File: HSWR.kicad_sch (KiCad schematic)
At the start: 25 parts, among them J1 IO, J10 W2, J2 USB_B, J3 B+, J4 B-, J5 U1, J6 V1, J7 W1, J8 U2, J9 V2, U14 Opamp_Quad

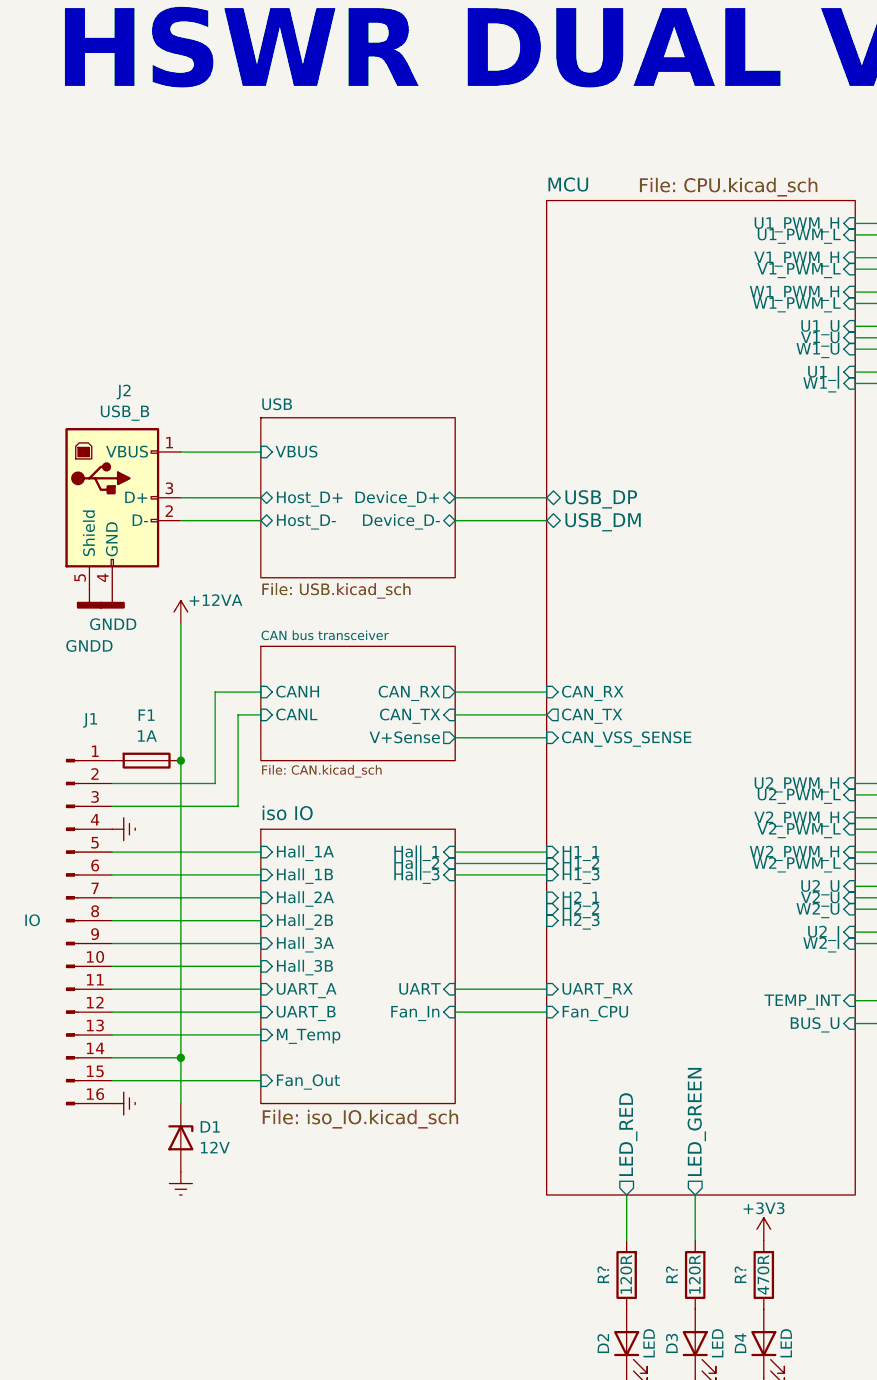
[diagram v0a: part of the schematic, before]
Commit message: - some layout work
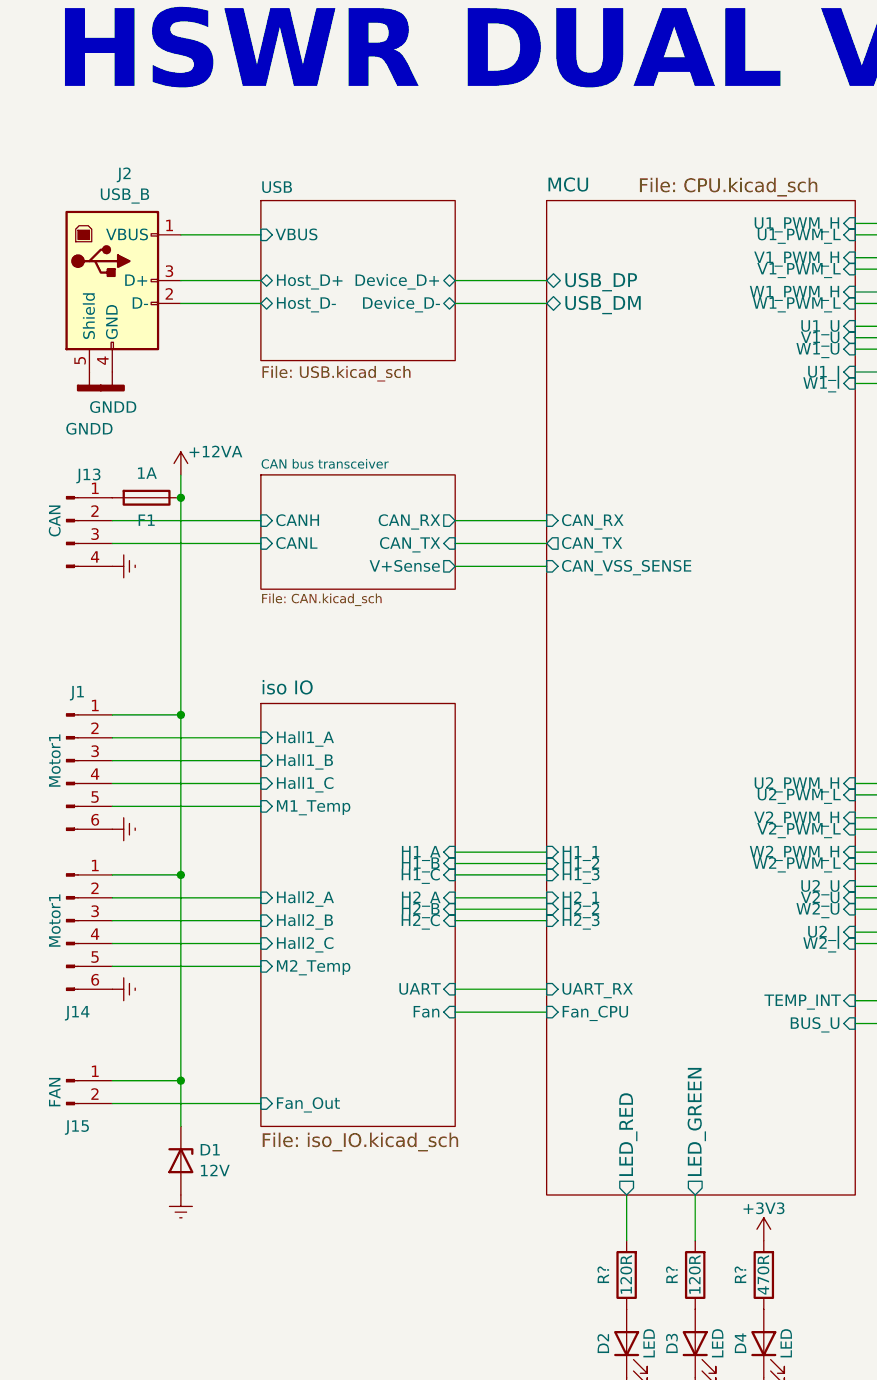
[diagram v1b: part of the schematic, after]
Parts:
- added J13: CAN, Connector_Phoenix_MC:PhoenixContact_MCV_1,5_4-G-3.5_1x04_P3.50mm_Vertical, symbol Connector:Conn_01x04_Pin
- added J14: Motor1, Connector_Phoenix_MC:PhoenixContact_MCV_1,5_6-G-3.5_1x06_P3.50mm_Vertical, symbol Connector:Conn_01x06_Pin
- added J15: FAN, Connector_Phoenix_MC:PhoenixContact_MCV_1,5_2-G-3.5_1x02_P3.50mm_Vertical, symbol Connector:Conn_01x02_Pin
- J1: value IO -> Motor1; footprint Connector_IDC:IDC-Header_2x08_P2.54mm_Vertical_Lock -> Connector_Phoenix_MC:PhoenixContact_MCV_1,5_6-G-3.5_1x06_P3.50mm_Vertical; symbol HSWR-rescue:Conn_01x16_Male-Connector -> Connector:Conn_01x06_Pin
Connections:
- net iso IO/Hall_1B is gone; now on net Earth: J1.6 (Pin_6)
- net +12VA: now also J1.1 (Pin_1), J14.1 (Pin_1), J15.1 (Pin_1); no longer J1.14 (Pin_14)
- net CAN bus transceiver/CANH: now also J13.2 (Pin_2); no longer J1.2 (Pin_2)
- net CAN bus transceiver/CANL: now also J13.3 (Pin_3); no longer J1.3 (Pin_3)
- net Earth: now also J13.4 (Pin_4), J14.6 (Pin_6); no longer J1.16 (Pin_16), J1.4 (Pin_4)
- net iso IO/Fan_Out: now also J15.2 (Pin_2); no longer J1.15 (Pin_15)
- net at F1.2: now also J13.1 (Pin_1); no longer J1.1 (Pin_1)
- net iso IO/Hall_1A renamed iso IO/M1_Temp
- removed net iso IO/Hall_2A: J1.7 (Pin_7)
- removed net iso IO/Hall_2B: J1.8 (Pin_8)
- removed net iso IO/Hall_3A: J1.9 (Pin_9)
- removed net iso IO/Hall_3B: J1.10 (Pin_10)
- removed net iso IO/M_Temp: J1.13 (Pin_13)
- removed net iso IO/UART_A: J1.11 (Pin_11)
- removed net iso IO/UART_B: J1.12 (Pin_12)
- new net iso IO/Hall1_A: J1.2 (Pin_2)
- new net iso IO/Hall1_B: J1.3 (Pin_3)
- new net iso IO/Hall1_C: J1.4 (Pin_4)
- new net iso IO/Hall2_A: J14.2 (Pin_2)
- new net iso IO/Hall2_B: J14.3 (Pin_3)
- new net iso IO/Hall2_C: J14.4 (Pin_4)
- new net iso IO/M2_Temp: J14.5 (Pin_5)
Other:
- sheet iso IO ports: added Fan, H1_A, H1_B, H1_C, H2_A, H2_B, H2_C, Hall1_A, Hall1_B, Hall1_C, Hall2_A, Hall2_B, Hall2_C, M1_Temp, M2_Temp; removed Fan_In, Hall_1, Hall_1A, Hall_1B, Hall_2, Hall_2A, Hall_2B, Hall_3, Hall_3A, Hall_3B, M_Temp, UART_A, UART_B
- moved on the sheet: D1, F1, J2
